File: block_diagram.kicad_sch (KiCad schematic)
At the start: 0 parts

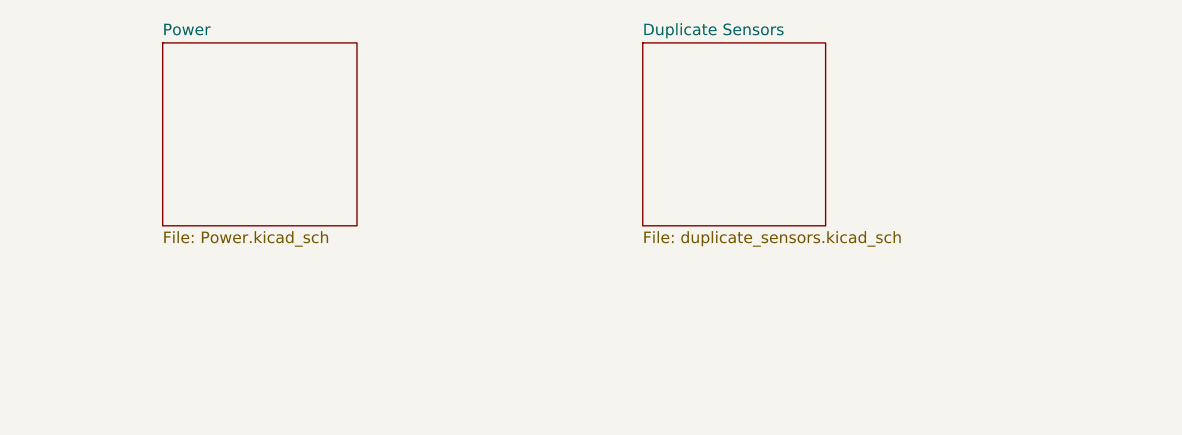
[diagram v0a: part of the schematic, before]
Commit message: Revert "Merge branch 'main' of https://github.com/pequeno212/PCB_SeniorDesign_team20"
This reverts commit 8ddd870afa6ea88a1f78691f7845b0b29e49b9ae, reversing
changes made to b7b9844e80cb26773f88e7278ccd95378529a98d.
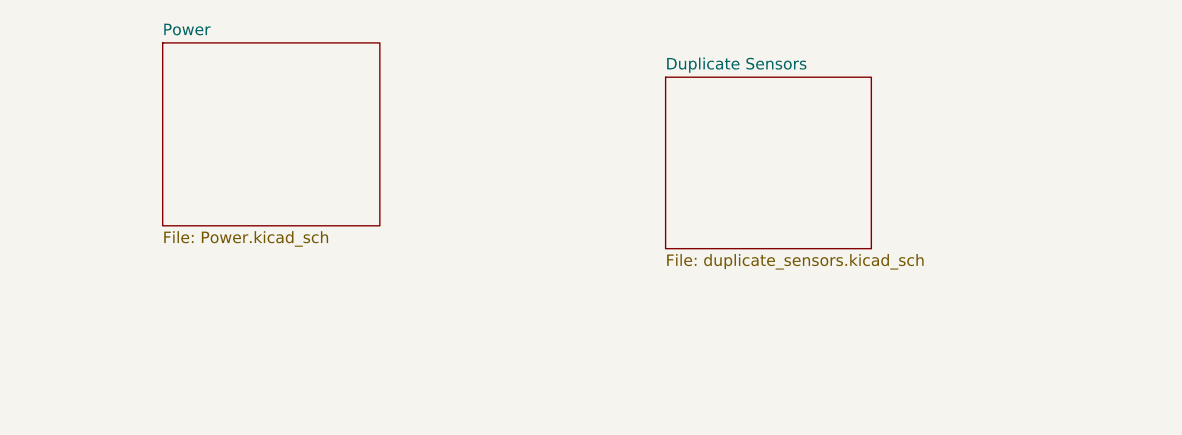
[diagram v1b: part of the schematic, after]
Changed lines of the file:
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@@
 	)
 	(sheet
-		(at 153.67 30.48)
-		(size 20.32 20.32)
+		(at 156.21 34.29)
+		(size 22.86 19.05)
 		(exclude_from_sim no)
 		(in_bom yes)
@@
 		)
 		(property "Sheetname" "Duplicate Sensors"
-			(at 153.67 29.7684 0)
+			(at 156.21 33.5784 0)
 			(show_name no)
 			(do_not_autoplace no)
@@
 		)
 		(property "Sheetfile" "duplicate_sensors.kicad_sch"
-			(at 153.67 51.3846 0)
+			(at 156.21 53.9246 0)
 			(show_name no)
 			(do_not_autoplace no)
@@
 	(sheet
 		(at 100.33 30.48)
-		(size 21.59 20.32)
+		(size 24.13 20.32)
 		(exclude_from_sim no)
 		(in_bom yes)
